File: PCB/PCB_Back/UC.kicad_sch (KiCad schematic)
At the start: 39 parts, among them J1 Sensor connector, J2 USB_C_Receptacle_USB2.0, J3 Lipo connector, Q1 UMH3N, Q2 PMOS, SW1 SW_Push_Dual, U1 ESP-12E, U2 CH340C, U3 MCP73831-2-OT, U4 MCP1700x-330xxTT, U6 BME680

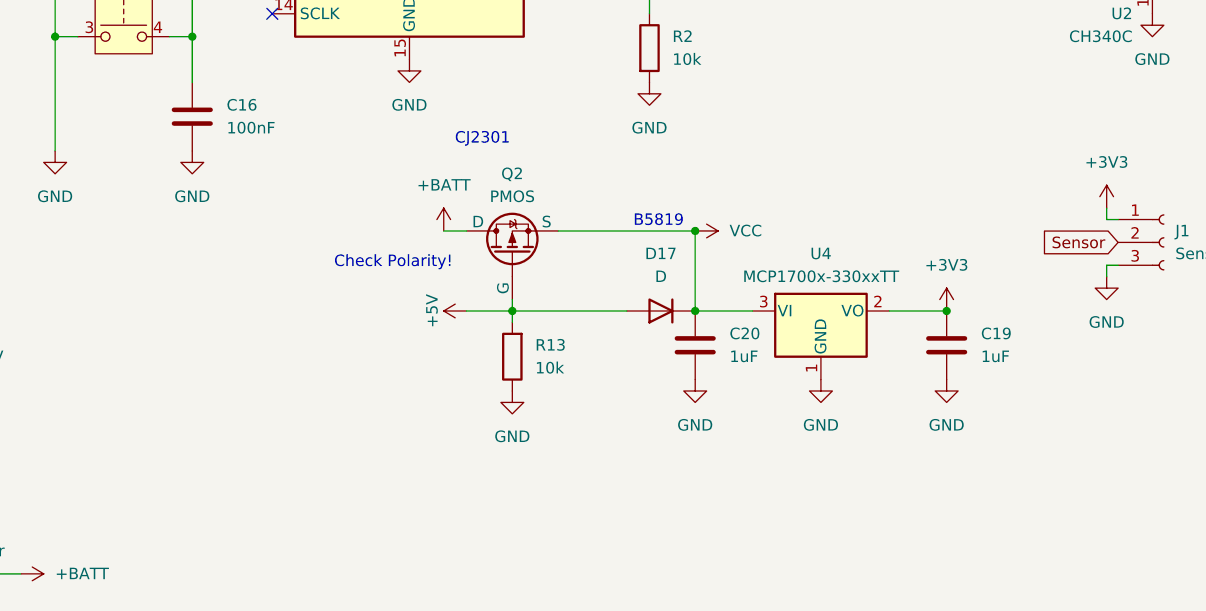
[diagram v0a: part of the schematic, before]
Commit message: Misc. Fixes, v1.0.
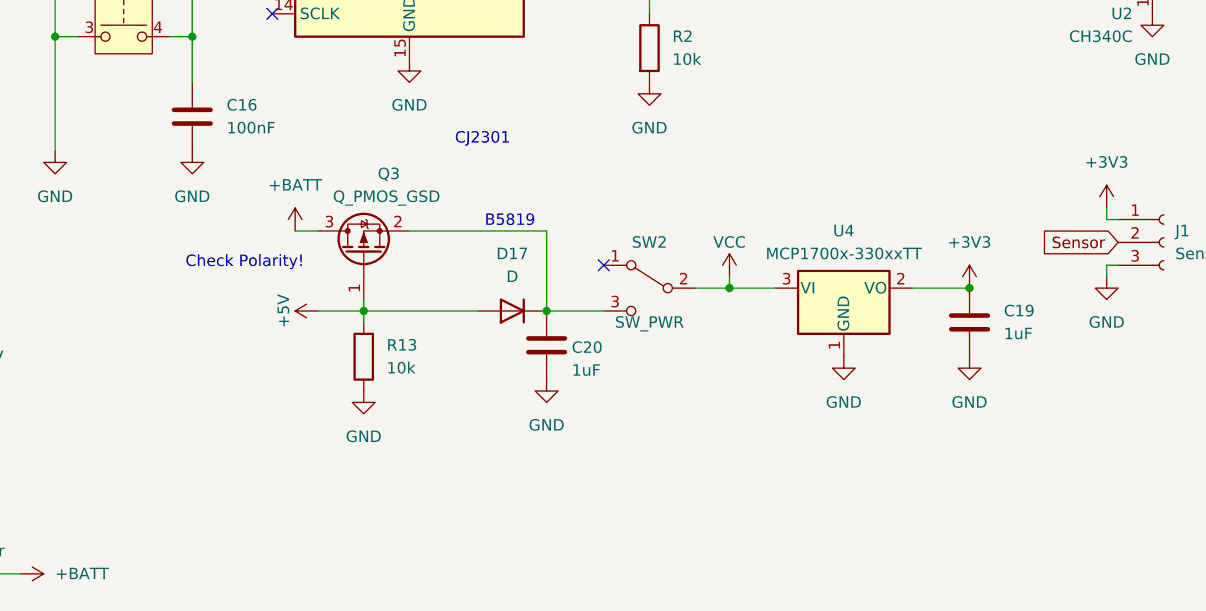
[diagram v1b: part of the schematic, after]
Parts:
- removed Q2: PMOS, Package_TO_SOT_SMD:SOT-23, symbol Simulation_SPICE:PMOS
- added Q3: Q_PMOS_GSD, Package_TO_SOT_SMD:SOT-23, symbol Device:Q_PMOS_GSD
- added SW2: SW_PWR, easyeda2kicad:SW-SMD_MK-12C02-G025, symbol Switch:SW_SPDT
- D16: footprint LED_SMD:LED_0805_2012Metric -> LED_SMD:LED_1206_3216Metric
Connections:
- net +5V: now also Q3.1 (G)
- net +BATT: now also Q3.3 (D)
- net VCC: now also SW2.2 (B); no longer C20.1, D17.1 (K)
- new net: C20.1, D17.1 (K), Q3.2 (S), SW2.3 (C)
- no-connect marks 17 -> 18
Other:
- moved on the sheet: C19, C20, D17, R13, U4
